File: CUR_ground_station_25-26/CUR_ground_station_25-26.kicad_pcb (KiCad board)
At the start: 2 copper layers, 81 parts, among them J1 Conn_01x02, J2 UJ20-C-H-G-SMT-P16-TR, J3 Conn_Coaxial_Small, J4 Conn_01x04_Pin, Q1 NTR4003N, Q2 NTR4003N, SW1 PTS815SJM250SMTRLFS, SW2 PTS815SJM250SMTRLFS, SW3 PTS815SJM250SMTRLFS, SW4 PTS815SJM250SMTRLFS, SW5 PTS815SJM250SMTRLFS, SW7 PTS815SJM250SMTRLFS, SW8 PTS815SJM250SMTRLFS, U1 ESP32-S3-MINI-1, U2 BQ24232RGT, U3 NCP186AMX330TAG, U4 USBLC6-2SC6, U5 E22-400MM_22S, U6 2.13" Epaper Module

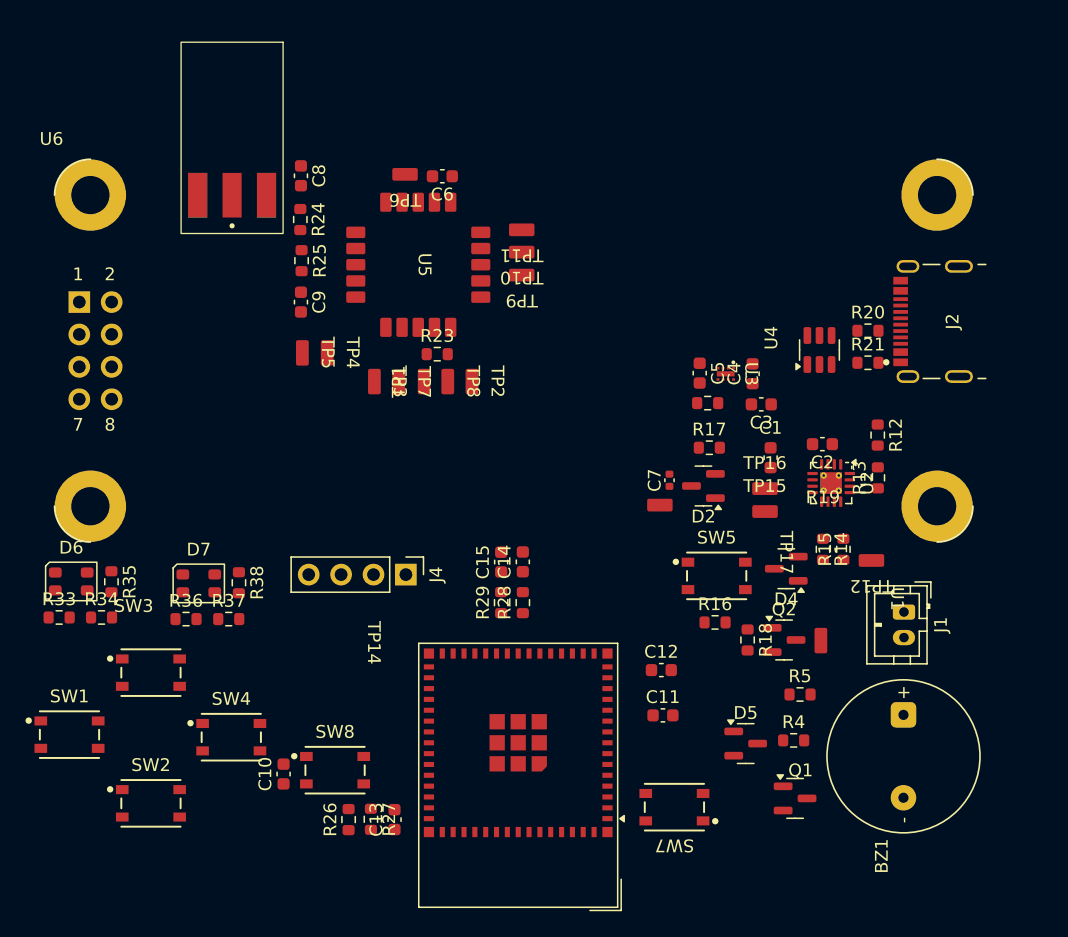
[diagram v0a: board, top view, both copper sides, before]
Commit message: layout
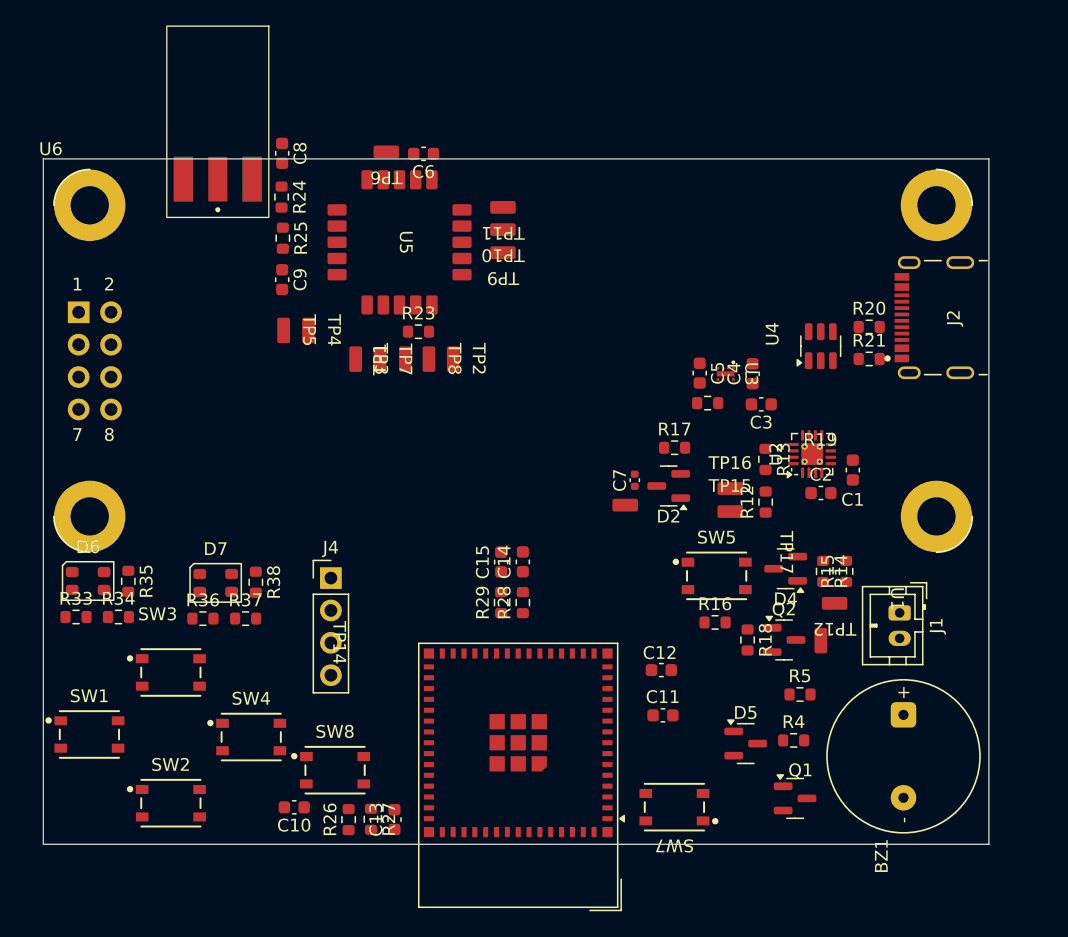
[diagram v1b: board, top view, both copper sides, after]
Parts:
- moved R12 10.2 mm to (104.7, 76.8), turned to 90 degrees
- moved R13 8.93 mm to (104.7, 73.5), turned to -90 degrees
- moved C1 6.52 mm to (111.6, 74.3), turned to -90 degrees
- moved J4 5.89 mm to (70.7, 82.8), turned to 0 degrees
- moved TP12 4.43 mm to (110.2, 84.8)
- moved C2 3.83 mm to (109.1, 76.1), turned to 0 degrees
- moved C10 2.74 mm to (67.8, 100.8), turned to 180 degrees
- moved TP14 2.72 mm to (93.7, 77.1)
- moved C7 2.72 mm to (94.5, 75.1)
- moved D2 2.72 mm to (97.1, 75.5)
- moved R17 2.72 mm to (97.6, 72.6)
- moved TP15 2.72 mm to (102.0, 77.6)
- moved TP16 2.72 mm to (102.0, 75.8)
- moved U2 2.72 mm to (108.4, 73.0), turned to 90 degrees
- moved TP5 2.29 mm to (66.9, 63.4)
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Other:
- board outline added: 74.2 x 53.8 mm

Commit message: Power layout
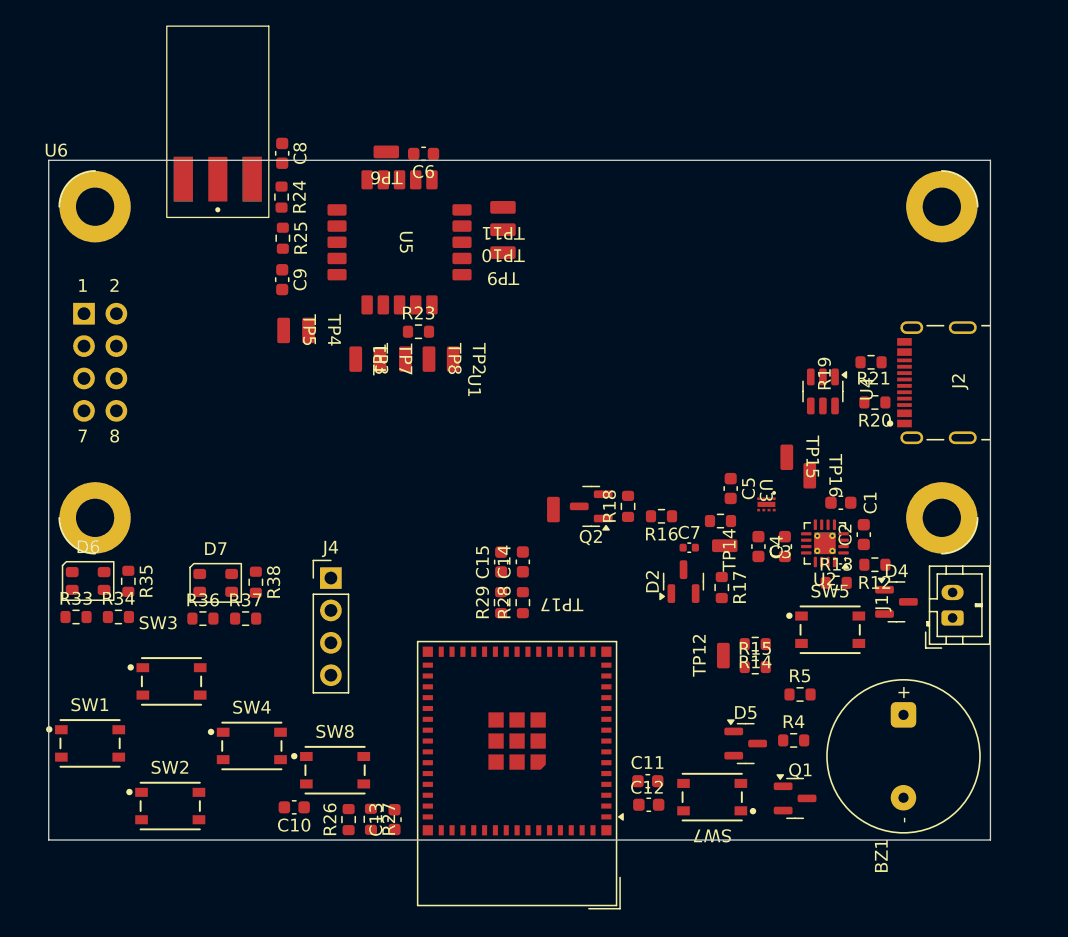
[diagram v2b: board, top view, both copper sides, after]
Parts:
- moved TP17 23.4 mm to (88.1, 77.4), turned to 90 degrees
- moved Q2 18.4 mm to (91.1, 77.2), turned to 180 degrees
- moved R18 14.1 mm to (94.0, 77.2), turned to 90 degrees
- moved C4 13.6 mm to (104.2, 80.3), turned to -90 degrees
- moved R17 11.6 mm to (101.3, 83.5), turned to -90 degrees
- moved C3 11.3 mm to (106.2, 80.3), turned to -90 degrees
- moved R13 11.2 mm to (110.3, 83.2), turned to 0 degrees
- moved U3 10.7 mm to (104.8, 77.0)
- moved C12 10.6 mm to (95.6, 100.5)
- moved R15 10.3 mm to (103.9, 89.8), turned to 0 degrees
- moved R12 9.88 mm to (113.3, 81.7), turned to 180 degrees
- moved SW5 9.85 mm to (109.8, 86.8)
- moved TP12 9.64 mm to (101.4, 88.8), turned to 90 degrees
- moved C5 9.37 mm to (102.0, 75.8)
- moved R16 9.32 mm to (96.6, 77.9), turned to 180 degrees
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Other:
- board size 74.2 x 53.8 mm -> 73.9 x 53.3 mm

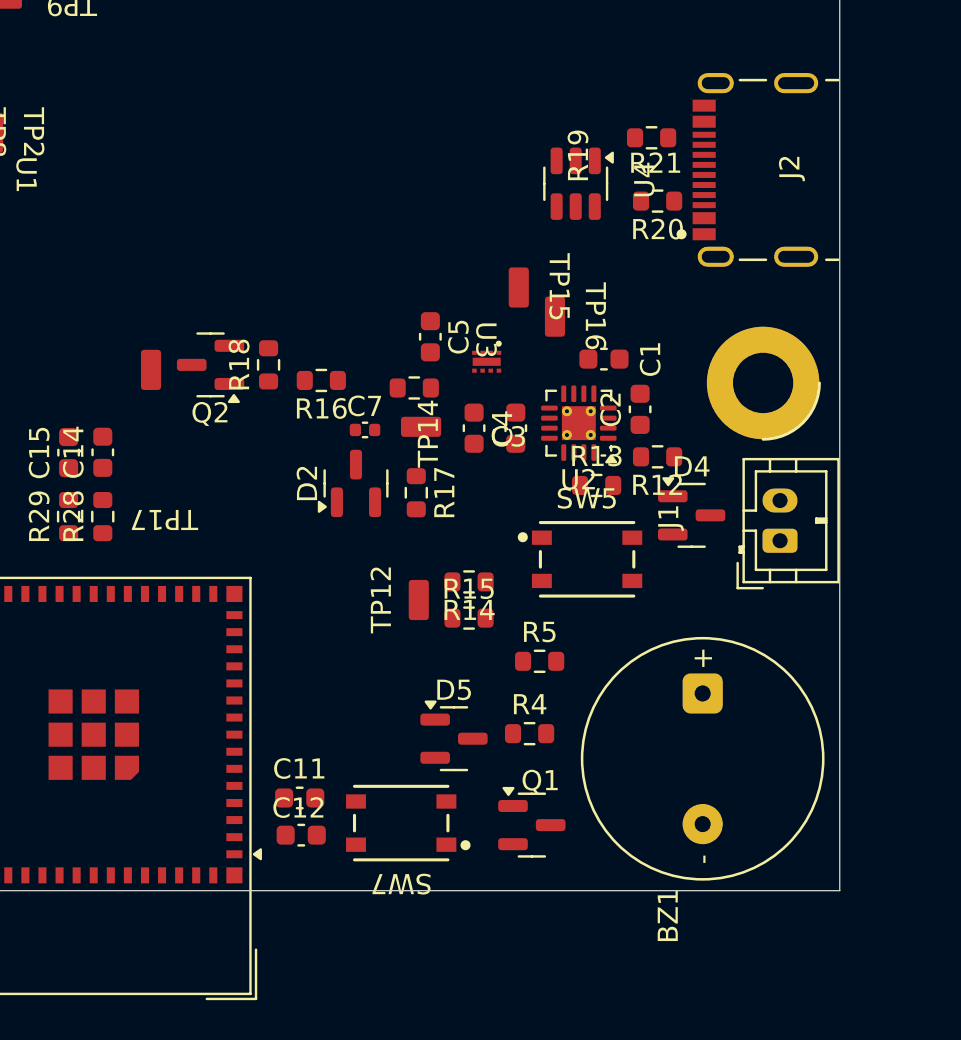
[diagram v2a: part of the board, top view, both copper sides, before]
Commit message: Update CUR_ground_station_25-26.kicad_pcb
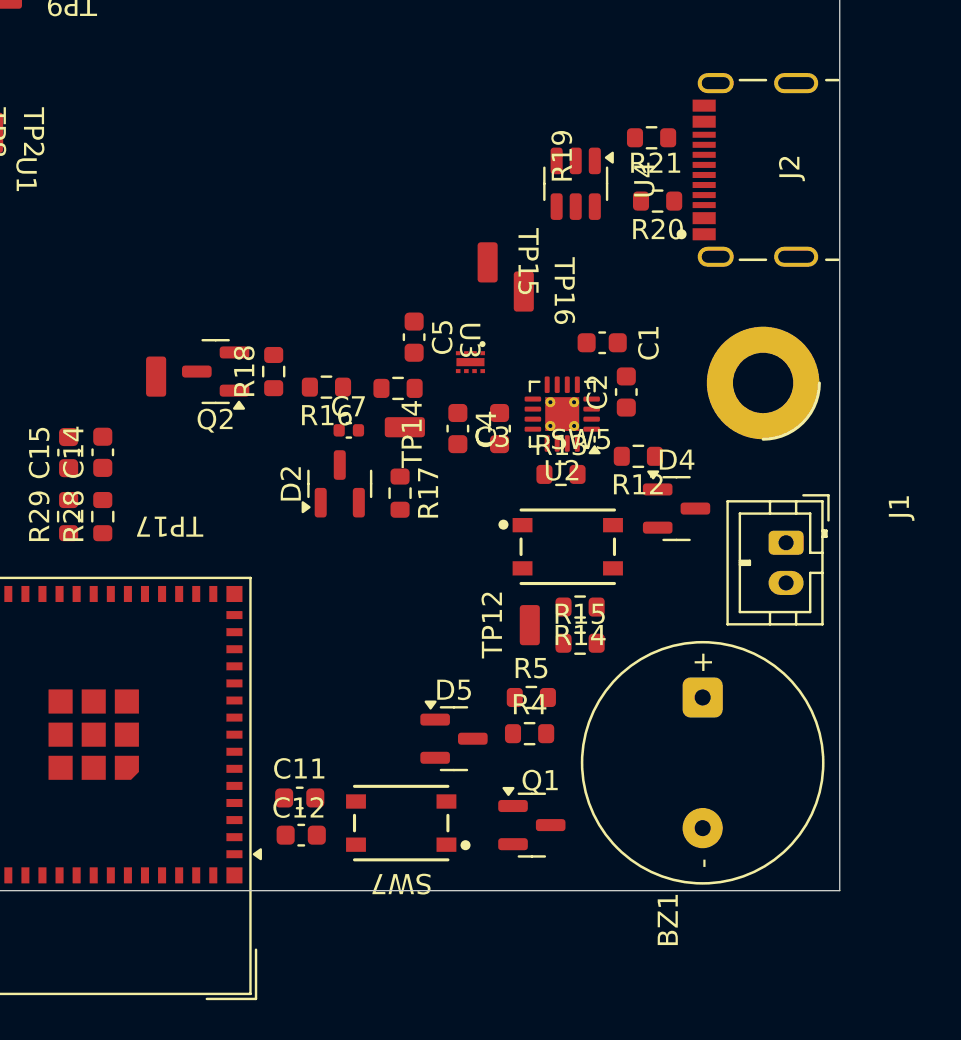
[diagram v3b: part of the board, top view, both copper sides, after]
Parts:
- moved R14 5.66 mm to (109.5, 89.2)
- moved R15 5.66 mm to (109.5, 91.0)
- moved TP12 5.66 mm to (107.0, 90.1)
- moved TP15 1.99 mm to (104.8, 72.0)
- moved TP16 1.99 mm to (106.7, 73.5)
- moved R13 1.86 mm to (108.5, 82.6)
- moved R5 1.85 mm to (107.0, 93.7)
- moved SW5 1.15 mm to (108.8, 86.2)
- moved C2 1.10 mm to (111.8, 78.5)
- moved R12 0.96 mm to (112.3, 81.7)
- moved U2 0.94 mm to (108.6, 79.6)
- moved D4 0.82 mm to (114.2, 84.3)
- moved C1 0.82 mm to (110.5, 76.0)
- moved C3 0.81 mm to (105.4, 80.3)
- moved C5 0.81 mm to (101.2, 75.8)
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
